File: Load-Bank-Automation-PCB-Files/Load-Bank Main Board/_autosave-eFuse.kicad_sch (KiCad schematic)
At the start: 29 parts, among them U1 TPS16411DRCR

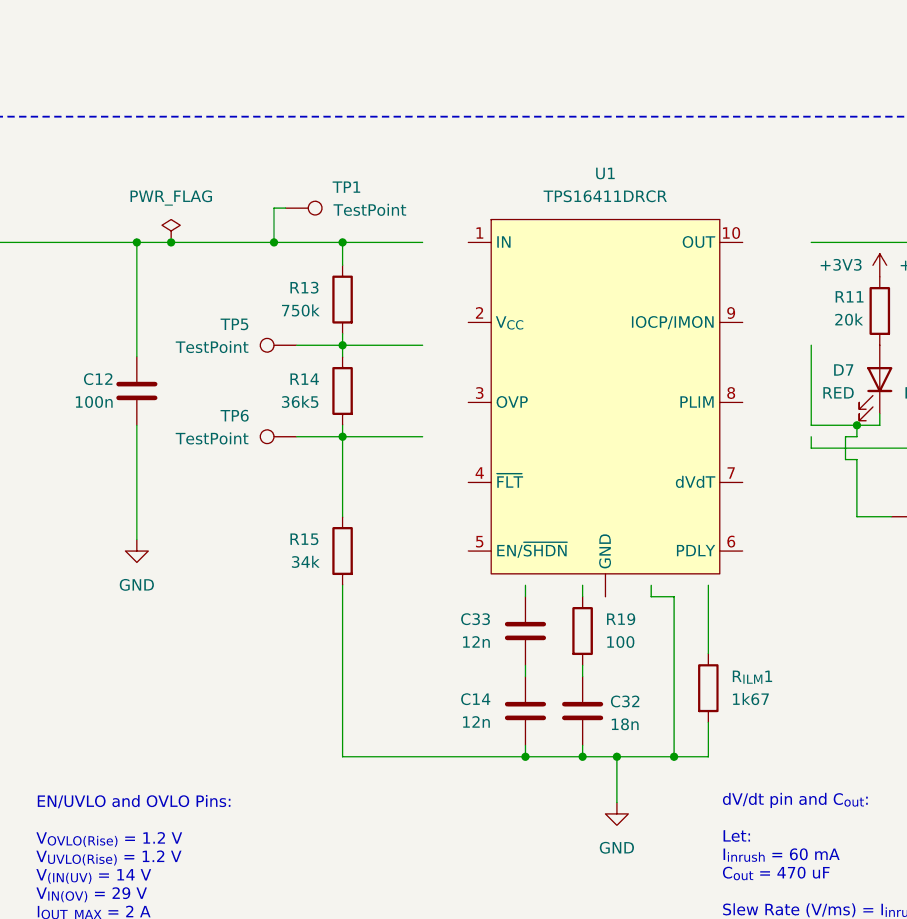
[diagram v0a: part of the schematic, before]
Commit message: A
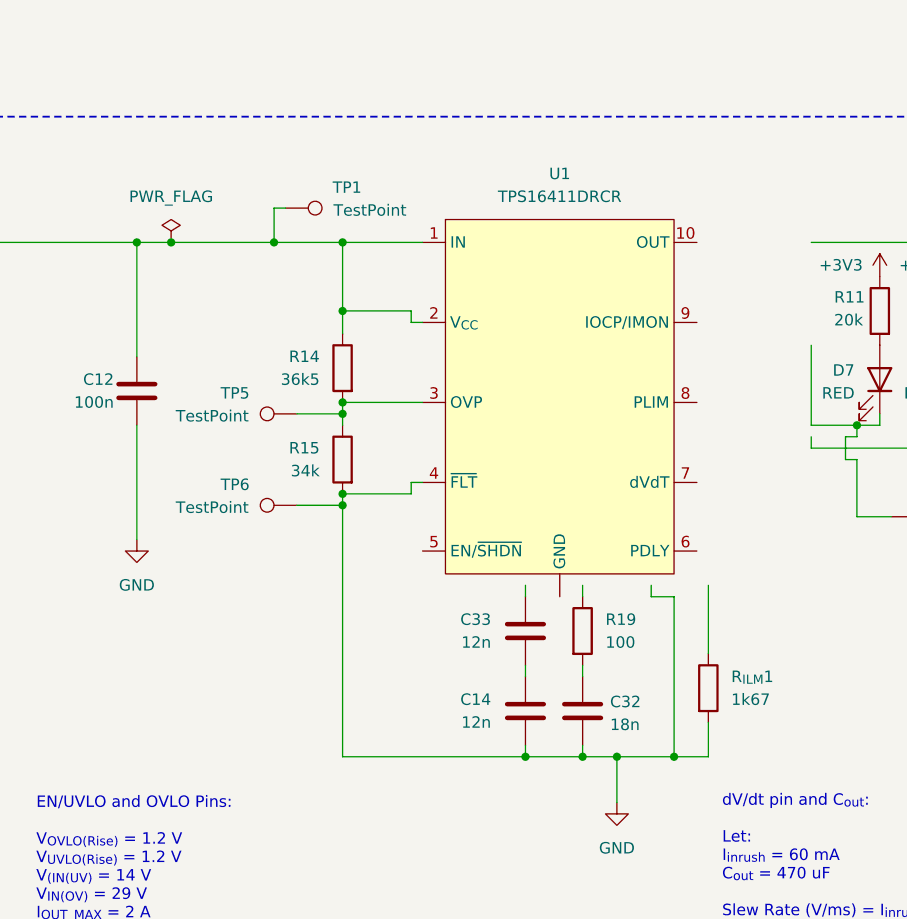
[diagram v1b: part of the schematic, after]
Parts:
- removed R13: 750k, Resistor_SMD:R_0805_2012Metric_Pad1.20x1.40mm_HandSolder, symbol Device:R
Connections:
- net GND: now also TP6.1, U1.4 (~{FLT})
- net Unprotected_19V: now also R14.1, U1.1 (IN), U1.2 (V_{CC})
- net at U1.3 (OVP): now also R14.2, R15.1, TP5.1
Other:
- moved on the sheet: R14, R15, TP5, TP6, U1
